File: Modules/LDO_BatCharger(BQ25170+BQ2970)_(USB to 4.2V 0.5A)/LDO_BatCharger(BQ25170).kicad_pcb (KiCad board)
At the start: 2 copper layers, 22.9 x 15.6 mm, 27 parts, among them J1 Conn_01x01, J2 Conn_01x01, J3 Conn_01x01, J4 Conn_01x01, J5 Conn_01x01, J7 Conn_01x01, J9 Conn_01x01, U1 BQ25170, U3 CSD16406Q3, U4 CSD16406Q3, U5 BQ2970

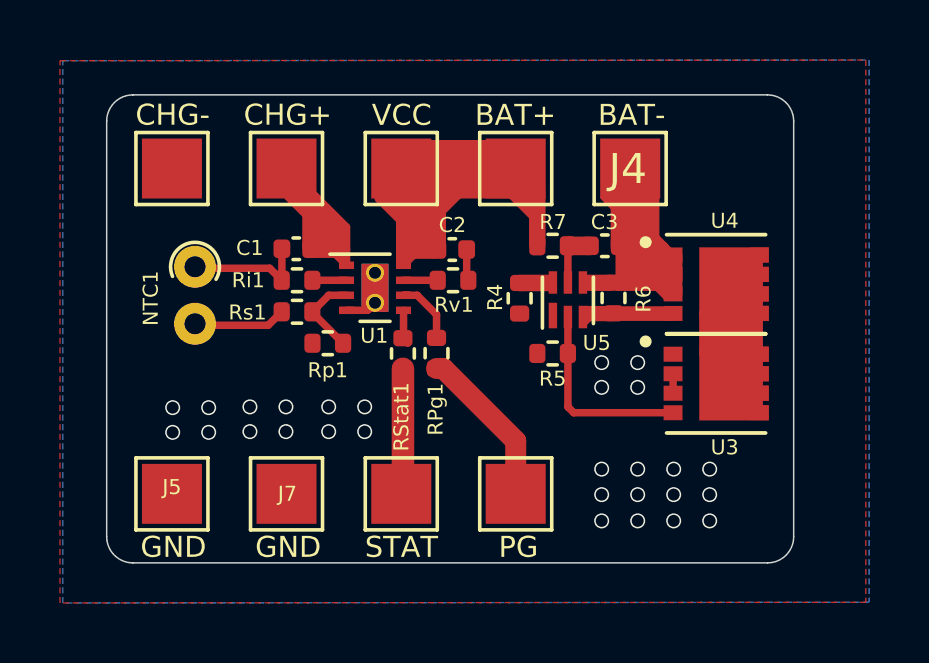
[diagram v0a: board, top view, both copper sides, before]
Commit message: Sort Out
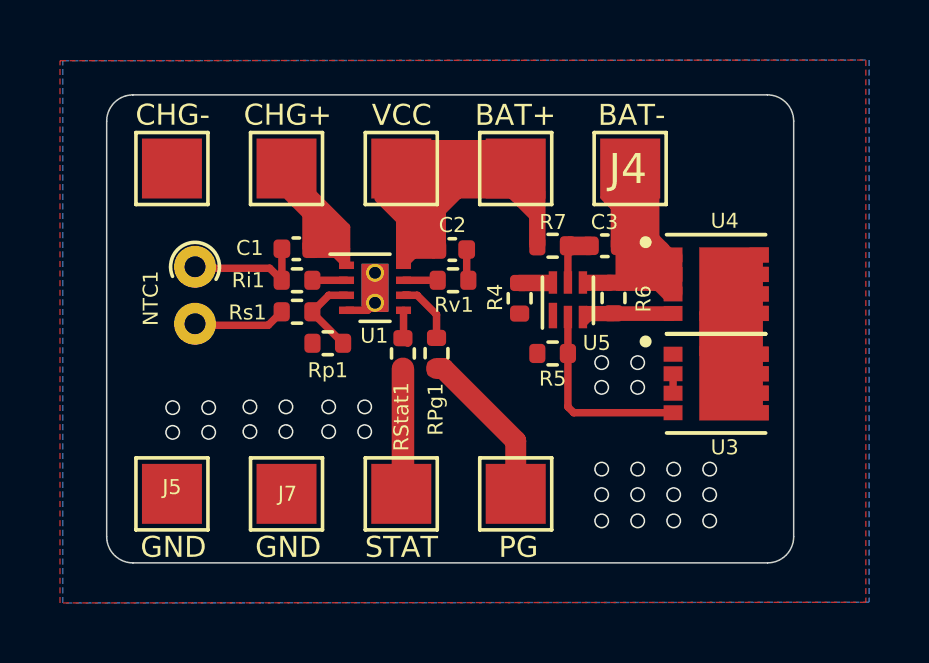
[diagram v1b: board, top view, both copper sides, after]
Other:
- net class Default removed
